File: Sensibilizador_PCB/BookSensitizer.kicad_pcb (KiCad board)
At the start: 2 copper layers, 100 x 100 mm, 37 parts, among them J1 Jack_out, J2 Jack_in, J3 Conn_inputs, M1 Fan, Q1 IRF630, Q2 IRF630, Q3 IRF630, Q4 IRF630, Q5 SI2302, U1 LM5104M, U2 LM5104M

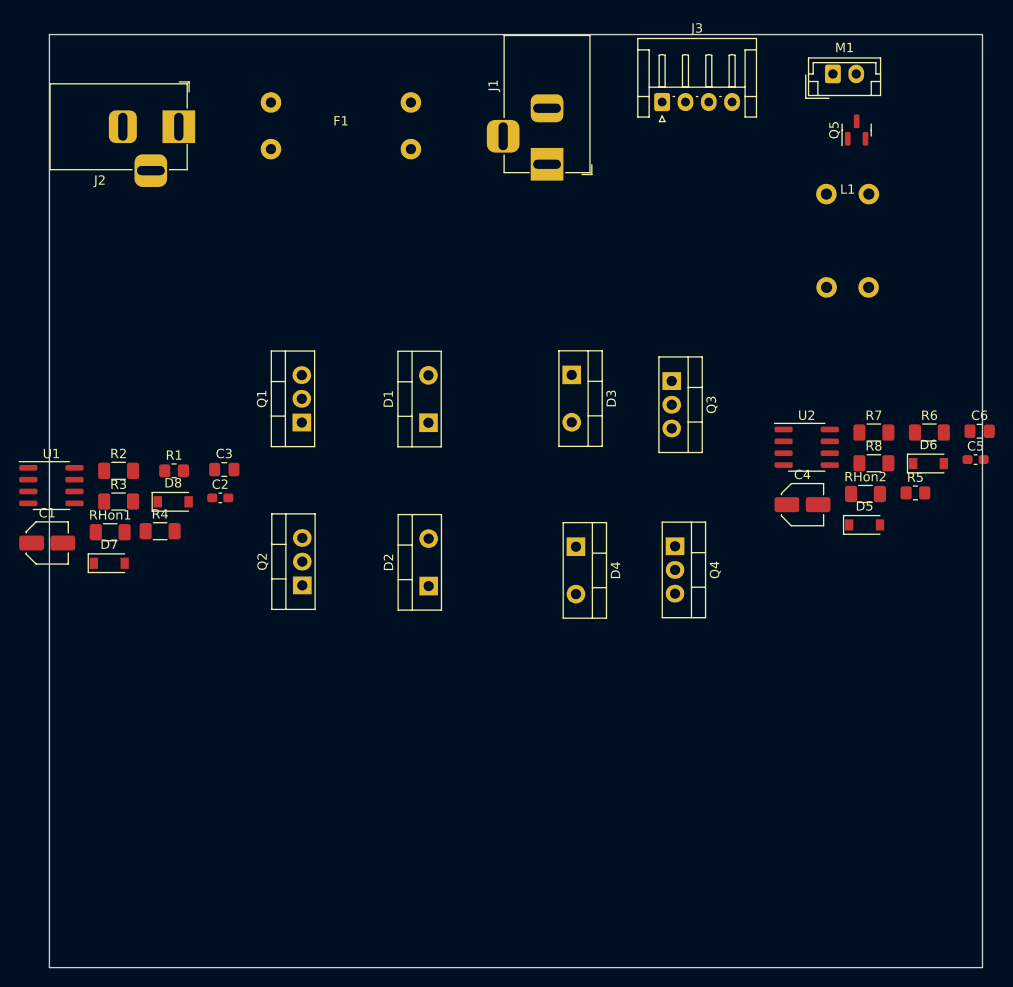
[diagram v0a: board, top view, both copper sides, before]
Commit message: Organizado 0 aire
0 aire
ready pa rutear
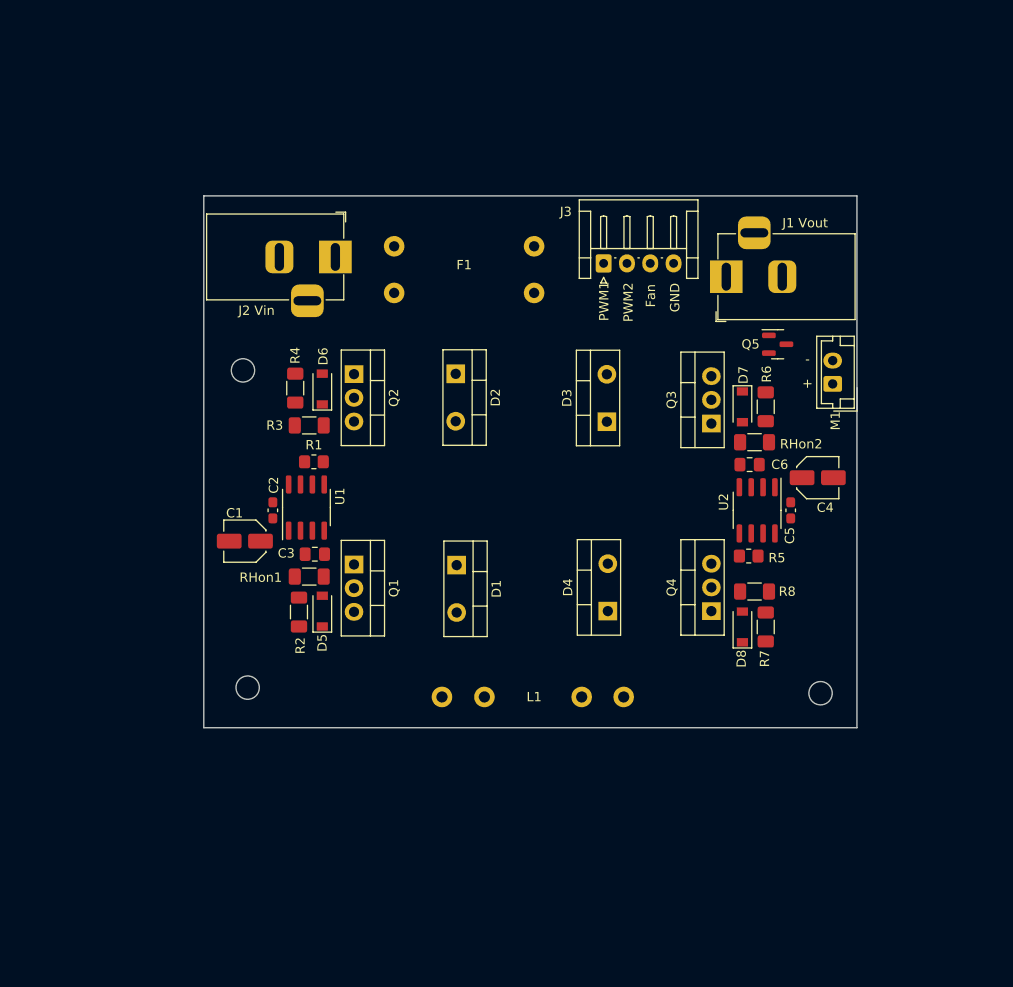
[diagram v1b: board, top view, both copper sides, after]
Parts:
- added REF**: MountingHole_2.5mm, MountingHole:MountingHole_2.5mm, F.Cu at (113.1, 88.9)
- added REF**: MountingHole_2.5mm, MountingHole:MountingHole_2.5mm, F.Cu at (175.0, 123.5)
- added REF**: MountingHole_2.5mm, MountingHole:MountingHole_2.5mm, F.Cu at (113.6, 122.9)
- J1 Vout: renamed from J1
- J2 Vin: renamed from J2
- moved D7 69.9 mm to (166.6, 92.8), turned to -90 degrees
- moved L1 67.8 mm to (136.7, 123.9)
- moved D6 65.5 mm to (121.6, 90.9), turned to 90 degrees
- moved D8 62.5 mm to (166.6, 116.4), turned to 90 degrees
- moved D5 58.8 mm to (121.6, 114.7), turned to 90 degrees
- moved M1 33.2 mm to (176.3, 90.3), turned to 90 degrees
- moved U1 27.4 mm to (119.9, 103.6), turned to 90 degrees
- moved C6 24.9 mm to (167.4, 99.0), turned to 180 degrees
- moved R2 24.6 mm to (119.1, 114.8), turned to -90 degrees
- moved Q5 24.5 mm to (170.4, 86.1), turned to 0 degrees
- moved R7 23.8 mm to (169.1, 116.4), turned to -90 degrees
- moved Q2 23.3 mm to (125.0, 89.3), turned to -90 degrees
- moved D2 22.9 mm to (135.9, 89.3), turned to -90 degrees
- moved J1 Vout 22.7 mm to (164.9, 78.9), turned to 180 degrees
- moved R3 22.0 mm to (120.2, 94.8)
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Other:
- board size 100 x 100 mm -> 70 x 57 mm
- board text added: "+"
- board text added: "-"
- board text added: "Fan"
- board text added: "GND"
- board text added: "PWM1"
- board text added: "PWM2"
